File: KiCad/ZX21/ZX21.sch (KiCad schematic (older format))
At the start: 46 parts, among them IC1 ULA 2C210E, IC2 AT28C256, IC3 Z80A, IC4 62256, J1 Jack-DC

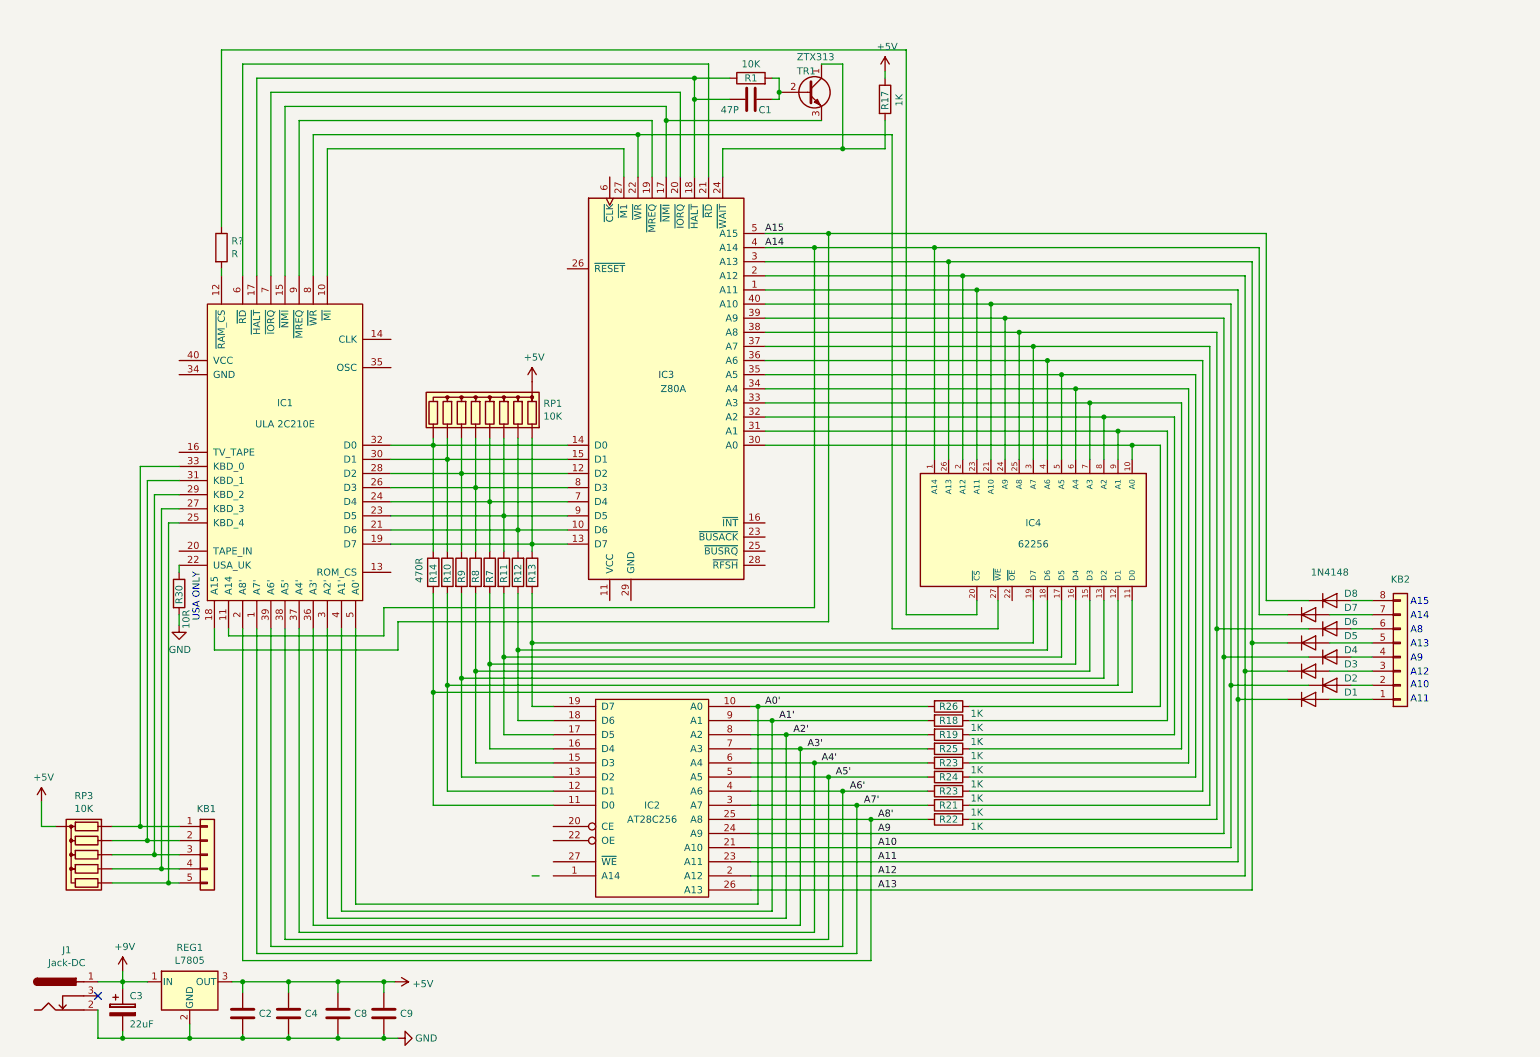
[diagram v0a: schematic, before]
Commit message: Main Sheet complete
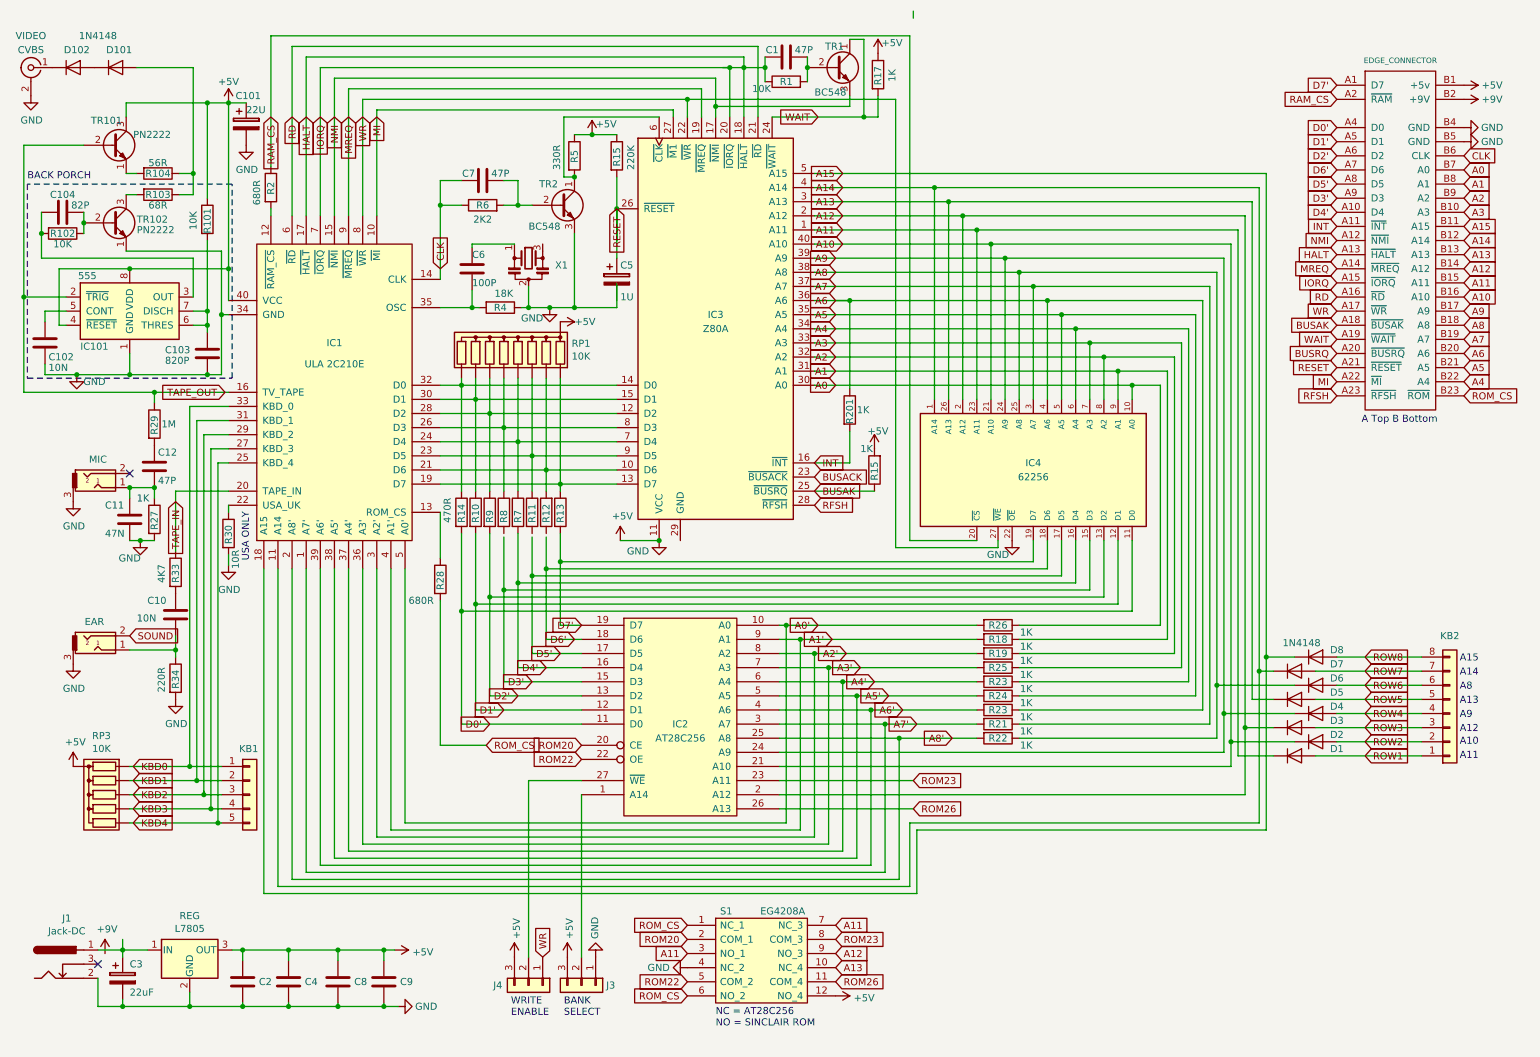
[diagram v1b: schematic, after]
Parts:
- added C10, C102: 10N, symbol device:C
- added C101: 22U, symbol device:CP
- added C103: 820P, symbol device:C
- added C104: 82P, symbol device:C
- added C11: 47N, symbol device:C
- added C12, C7: 47P, symbol device:C
- added C5: 1U, symbol device:CP
- added C6: 100P, symbol device:C
- added D101, D102: 1N4148, Diodes_THT:D_DO-35_SOD27_Horizontal_RM10, symbol Diode:1N4148
- added EAR, MIC: Audio-Jack-3, symbol Connector:Audio-Jack-3
- added EDGE_CONNECTOR: ZX81BUS, symbol Sinclair:ZX81BUS
- added IC101: 555, symbol Sinclair:TLC555
- added J3, J4: Conn_01x03, symbol Connector:Conn_01x03
- added R101, R102: 10K, symbol device:R
- added R103: 68R, symbol device:R
- added R104: 56R, symbol device:R
- added R15, R201, R27: 1K, symbol device:R
- added R15: 220K, symbol device:R
- added R28: 680R, symbol device:R
- added R29: 1M, symbol device:R
- added R33: 4K7, symbol device:R
- added R34: 220R, symbol device:R
- added R4: 18K, symbol device:R
- added R5: 330R, symbol device:R
- added R6: 2K2, symbol device:R
- added S1: EG4208A, EG4208A, symbol Sinclair:EG4208A
- added TR101, TR102: PN2222, TO_SOT_Packages_THT:TO-92_Molded_Narrow, symbol Transistor:PN2222A
- added TR2: BC548, TO_SOT_Packages_THT:TO-92_Molded_Narrow, symbol Transistor:BC548
- added VIDEO: CVBS, symbol Connector:Conn_Coaxial
- added X1: Resonator_Small, symbol device:Resonator_Small
- R2: renamed from R?; value R -> 680R
- TR1: value ZTX313 -> BC548
- renumbered REG1 to REG
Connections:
- net GND is gone; now on net +5V: C2.2, C3.2, C4.2, C8.2, C9.2, IC2.14 (GND), IC4.14 (GND), J1.2, R30.2, REG.2 (GND)
- net +5V: now also IC1.34 (GND), IC1.40 (VCC), IC3.11 (VCC), IC4.22 (~OE), C101.1, C101.2, C102.2, C103.2, C11.2, EAR.3, EDGE_CONNECTOR.B1 (+5v), EDGE_CONNECTOR.B4 (GND), EDGE_CONNECTOR.B5 (GND), IC101.1 (GND), IC101.4 (~RESET), IC101.8 (VDD), J3.1 (Pin_1), J3.3 (Pin_3), J4.3 (Pin_3), MIC.3, R101.1, R15.1, R15.2, R27.2, R34.2, R4.1, R5.1, S1.12 (NO_4), S1.4 (NC_2), TR101.3 (C), TR102.1 (E), TR2.3 (E), VIDEO.2 (Ext), X1.2
- net +9V: now also EDGE_CONNECTOR.B2 (+9V); no longer C3.1, J1.1, REG.1 (IN)
- net A10: now also EDGE_CONNECTOR.B16 (A10)
- net A11: now also EDGE_CONNECTOR.B15 (A11), S1.3 (NO_1), S1.7 (NC_3); no longer IC2.23 (A11)
- net A12: now also EDGE_CONNECTOR.B14 (A12), S1.9 (NO_3)
- net A13: now also EDGE_CONNECTOR.B13 (A13), S1.10 (NC_4); no longer IC2.26 (A13)
- net A14: now also EDGE_CONNECTOR.B12 (A14)
- net A15: now also EDGE_CONNECTOR.B11 (A15)
- net A9: now also EDGE_CONNECTOR.B17 (A9)
- net A0: now reaches IC3.30 (A0), IC4.10 (A0), R26.1
- net A0: now also EDGE_CONNECTOR.B7 (A0)
- net D0': now reaches IC2.11 (D0), IC4.11 (D0), R14.2
- net D0': now also EDGE_CONNECTOR.A4 (D0)
- net D1': now reaches IC2.12 (D1), IC4.12 (D1), R10.2
- net D1': now also EDGE_CONNECTOR.A5 (D1)
- net D2': now reaches IC2.13 (D2), IC4.13 (D2), R9.2
- net D2': now also EDGE_CONNECTOR.A6 (D2)
- net D3': now reaches IC2.15 (D3), IC4.15 (D3)
- net D3': now also EDGE_CONNECTOR.A9 (D3); no longer R8.2
- net D4': now reaches IC2.16 (D4), IC4.16 (D4), R7.2
- net D4': now also EDGE_CONNECTOR.A10 (D4)
- net D5': now reaches IC2.17 (D5), IC4.17 (D5)
- net D5': now also EDGE_CONNECTOR.A8 (D5); no longer R11.2
- net D6': now reaches IC2.18 (D6), IC4.18 (D6)
- net D6': now also EDGE_CONNECTOR.A7 (D6); no longer R12.1
- net D7': now reaches IC2.19 (D7), IC4.19 (D7), R13.2
- net D7': now also EDGE_CONNECTOR.A1 (D7)
- net RAM_CS: now reaches IC4.20 (~CS), R2.1
- net RAM_CS: now also EDGE_CONNECTOR.A2 (~RAM)
- net A8: now reaches D6.1 (K), IC3.38 (A8), IC4.25 (A8), R22.1
- net A8: now also EDGE_CONNECTOR.B18 (A8)
- net WR: now reaches IC1.8 (~WR), IC3.22 (~WR), IC4.27 (~WE)
- net WR: now also EDGE_CONNECTOR.A17 (~WR), J4.1 (Pin_1)
- net A7: now reaches IC3.37 (A7), IC4.3 (A7), R21.1
- net A7: now also EDGE_CONNECTOR.B19 (A7)
- net A6: now reaches IC3.36 (A6), IC4.4 (A6), R23.1
- net A6: now also EDGE_CONNECTOR.B20 (A6), R201.1
- net A5: now reaches IC3.35 (A5), IC4.5 (A5), R24.1
- net A5: now also EDGE_CONNECTOR.B21 (A5)
- net A4: now reaches IC3.34 (A4), IC4.6 (A4), R23.1
- net A4: now also EDGE_CONNECTOR.B22 (A4)
- net A3: now reaches IC3.33 (A3), IC4.7 (A3), R25.1
- net A3: now also EDGE_CONNECTOR.B10 (A3)
- net A2: now reaches IC3.32 (A2), IC4.8 (A2), R19.1
- net A2: now also EDGE_CONNECTOR.B9 (A2)
- net A1: now reaches IC3.31 (A1), IC4.9 (A1), R18.1
- net A1: now also EDGE_CONNECTOR.B8 (A1)
- net MI: now reaches IC1.10 (~MI), IC3.27 (~M1~)
- net MI: now also EDGE_CONNECTOR.A22 (~MI)
- net at IC1.13 (ROM_CS): now also R28.1
- net CLK: now reaches IC1.14 (CLK)
- net CLK: now also C7.2, EDGE_CONNECTOR.B6 (CLK), R6.1
- net NMI: now reaches IC1.15 (~NMI), IC3.17 (~NMI), TR1.3 (E)
- net NMI: now also EDGE_CONNECTOR.A12 (~NMI)
- net TAPE_OUT: now reaches IC1.16 (TV_TAPE)
- net TAPE_OUT: now also IC101.2 (~TRIG), R29.1, TR101.2 (B)
- net HALT: now reaches C1.2, IC1.17 (~HALT), IC3.18 (~HALT), R1.1
- net HALT: now also IC1.7 (~IORQ), IC3.20 (~IORQ), EDGE_CONNECTOR.A13 (~HALT), EDGE_CONNECTOR.A15 (~IORQ)
- net TAPE_IN: now reaches IC1.20 (TAPE_IN)
- net TAPE_IN: now also R33.1
- net KBD4: now reaches IC1.25 (KBD_4), KB1.5 (Pin_5), RP3.6 (R5)
- net KBD3: now reaches IC1.27 (KBD_3), KB1.4 (Pin_4), RP3.5 (R4)
- net KBD2: now reaches IC1.29 (KBD_2), KB1.3 (Pin_3), RP3.4 (R3)
- net KBD1: now reaches IC1.31 (KBD_1), KB1.2 (Pin_2), RP3.3 (R2)
- net KBD0: now reaches IC1.33 (KBD_0), KB1.1 (Pin_1), RP3.2 (R1)
- net at IC1.35 (OSC): now also C6.2, R4.2
- net RD: now reaches IC1.6 (~RD), IC3.21 (~RD)
- net RD: now also EDGE_CONNECTOR.A16 (~RD)
- net MREQ: now reaches IC1.9 (~MREQ), IC3.19 (~MREQ)
- net MREQ: now also EDGE_CONNECTOR.A14 (~MREQ)
- net INT: now reaches IC3.16 (~INT)
- net INT: now also EDGE_CONNECTOR.A11 (~INT), R201.2
- net BUSACK: now reaches IC3.23 (~BUSACK)
- net WAIT: now reaches IC3.24 (~WAIT~), R17.2, TR1.1 (C)
- net WAIT: now also EDGE_CONNECTOR.A19 (~WAIT)
- net BUSAK: now reaches IC3.25 (~BUSRQ)
- net BUSAK: now also EDGE_CONNECTOR.A18 (~BUSAK), R15.1
- net RESET: now reaches IC3.26 (~RESET)
- net RESET: now also C5.1, EDGE_CONNECTOR.A21 (~RESET), R15.2
- net RFSH: now reaches IC3.28 (~RFSH)
- net RFSH: now also EDGE_CONNECTOR.A23 (~RFSH)
- net at IC3.6 (~CLK): now also R5.2, TR2.1 (C)
- net at IC2.1 (A14): now also J3.2 (Pin_2)
- net ROM20: now reaches IC2.20 (CE)
- net ROM20: now also S1.2 (COM_1)
- net ROM22: now reaches IC2.22 (OE)
- net ROM22: now also S1.5 (COM_2)
- net at IC2.27 (~WE): now also J4.2 (Pin_2)
- net ROW1: now reaches D1.2 (A), KB2.1 (Pin_1)
- net ROW2: now reaches D2.2 (A), KB2.2 (Pin_2)
- net ROW3: now reaches D3.2 (A), KB2.3 (Pin_3)
- net ROW4: now reaches D4.2 (A), KB2.4 (Pin_4)
- net ROW5: now reaches D5.2 (A), KB2.5 (Pin_5)
- net ROW6: now reaches D6.2 (A), KB2.6 (Pin_6)
- net ROW7: now reaches D7.2 (A), KB2.7 (Pin_7)
- net ROW8: now reaches D8.2 (A), KB2.8 (Pin_8)
- new net: C3.1, J1.1, REG.1 (IN)
- new net: D102.1 (K), VIDEO.1 (In)
- new net: C104.1, IC101.3 (OUT), R102.2
- new net: C102.1, IC101.5 (CONT)
- new net: C103.1, IC101.6 (THRES), IC101.7 (DISCH), R101.2
- new net: D101.1 (K), D102.2 (A)
- new net: D101.2 (A), R103.1, R104.1
- new net: R104.2, TR101.1 (E)
- new net: R103.2, TR102.3 (C)
- new net: C104.2, R102.1, TR102.2 (B)
- new net: C7.1, R6.2, TR2.2 (B)
- new net: C10.2, EAR.1, R34.1
- new net: C11.1, C12.2, MIC.1, R27.1
- new net: C10.1, R33.2
- new net: C12.1, R29.2
- new net: C6.1, X1.1
- new net BUSRQ: EDGE_CONNECTOR.A20 (~BUSRQ)
- new net ROM23: IC2.23 (A11), S1.8 (COM_3)
- new net ROM26: IC2.26 (A13), S1.11 (COM_4)
- new net ROM_CS: EDGE_CONNECTOR.B23 (~ROM), R28.2, S1.1 (NC_1), S1.6 (NO_2)
- new net SOUND: EAR.2
- no-connect marks 1 -> 2
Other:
- note added: "A Top B Bottom"
- note added: "BACK PORCH"
- note added: "BANK\nSELECT"
- note added: "NC = AT28C256\nNO = SINCLAIR ROM"
- note added: "WRITE\nENABLE"
- moved on the sheet: C1, C2, C3, C4, C8, C9, D1, D2, D3, D4, D5, D6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
